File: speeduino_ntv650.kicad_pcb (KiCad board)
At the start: 2 copper layers, 101.6 x 96.5 mm, 70 parts, among them IC1 SP721, IC2 TC4424, J1 Conn_01x25_DB-25, P1 MAX9926_9927, Q1 STP62NS04Z, Q2 STP62NS04Z, Q3 STP62NS04Z, U1 LM2937xT

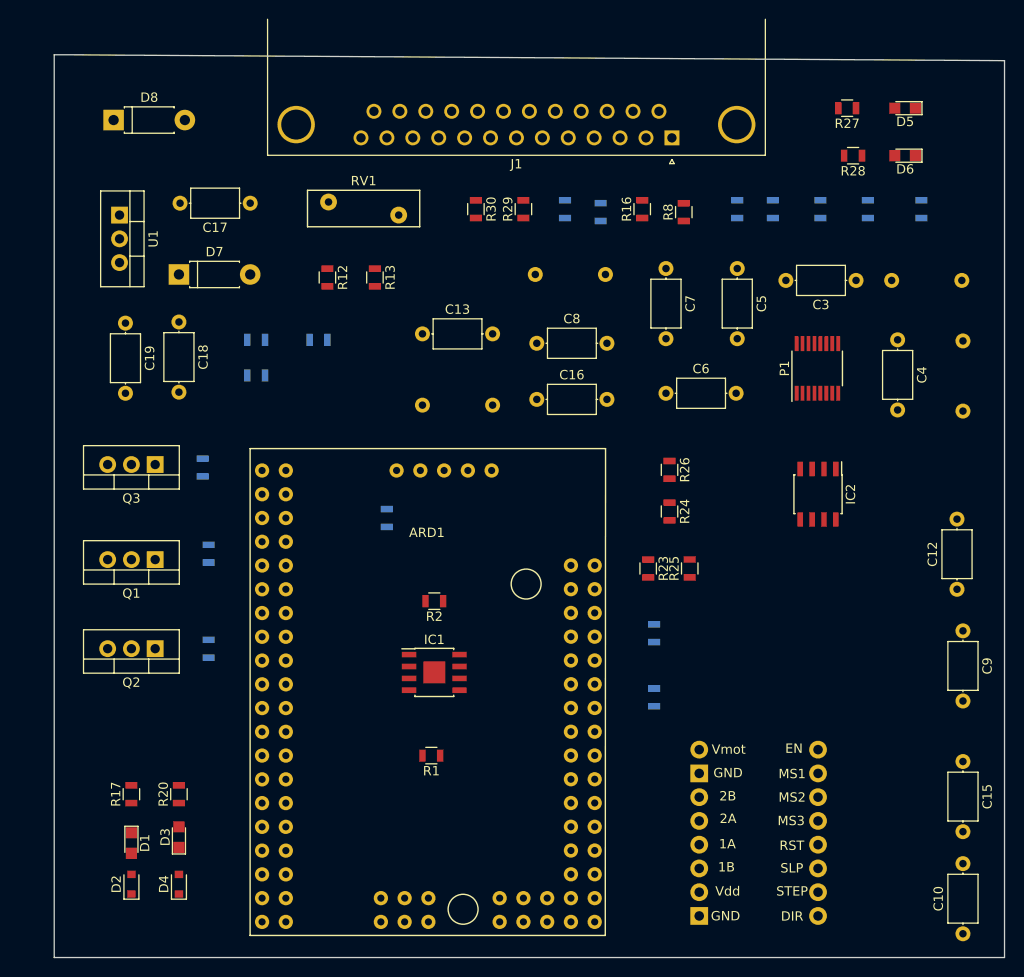
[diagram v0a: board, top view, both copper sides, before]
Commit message: change footprints
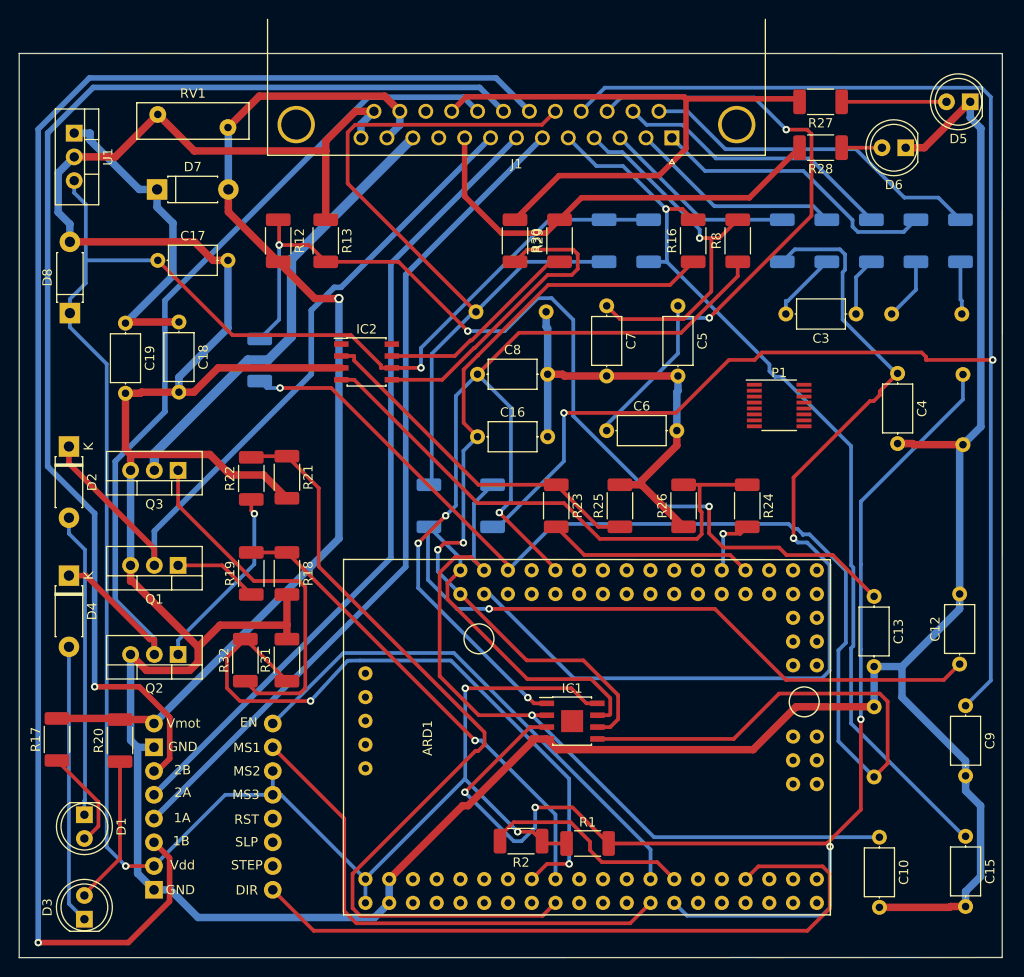
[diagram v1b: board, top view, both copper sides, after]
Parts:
- D1, D3, D5, D6: footprint LEDs:LED_0805 -> LED_THT:LED_D5.0mm
- D2, D4: footprint Diodes_SMD:D_0805 -> Diode_THT:D_DO-41_SOD81_P7.62mm_Horizontal
- R1, R10, R11, R12, R13, R14, R15, R16, R17, R2, R20, R23, R24, R25, R26, R27, R28, R29, R3, R30, R4, R5, R6, R7, R8, R9: footprint Resistors_SMD:R_0805 -> Resistor_SMD:R_2010_5025Metric
- R18, R19, R21, R22, R31, R32: footprint Resistors_SMD:R_0805 -> Resistor_SMD:R_2010_5025Metric; moved to F.Cu
- moved C14 62.5 mm to (151.8, 103.2), turned to 90 degrees
- moved A1 58.4 mm to (88.8, 96.3)
- moved C13 55.9 mm to (151.8, 83.9), turned to 270 degrees
- moved IC2 50.3 mm to (97.5, 58.9), turned to 0 degrees
- moved D2 47.3 mm to (65.7, 67.9), turned to 270 degrees
- moved D4 35.0 mm to (65.7, 81.7), turned to 270 degrees
- moved ARD1 31.0 mm to (99.9, 104.0), turned to 90 degrees
- moved R31 30.6 mm to (89.0, 90.8), turned to 90 degrees
- moved R11 27.7 mm to (104.2, 74.3)
- moved R2 27.3 mm to (114.0, 110.1)
- moved R9 26.8 mm to (111.0, 74.3)
- moved D8 21.2 mm to (65.8, 53.7), turned to 90 degrees
- moved R32 21.1 mm to (84.6, 90.8), turned to 90 degrees
- moved RV1 20.5 mm to (82.7, 33.8)
- moved R1 19.2 mm to (121.2, 110.4), turned to 0 degrees
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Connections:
- C17 pad 1: 12V -> 5V
- IC2 pad 6: 12V -> 5V
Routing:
- net GND: track 0.00 -> 485.5 mm
- net 5V: track 0.00 -> 240.8 mm, vias 0 -> 4
- net TPS_sens: track 0.00 -> 176.4 mm, vias 0 -> 2
- net STEP-1B-OUT: track 0.00 -> 166.1 mm, vias 0 -> 1
- net ADC-Clamp4: track 0.00 -> 141.6 mm, vias 0 -> 1
- net ADC-Clamp5: track 0.00 -> 137.6 mm, vias 0 -> 4
- net STEP-2B-OUT: track 0.00 -> 129.1 mm, vias 0 -> 1
- net 12V: track 0.00 -> 112.8 mm, vias 0 -> 1
- net ADC-Clamp1: track 0.00 -> 103.5 mm, vias 0 -> 4
- net Net-(C13-Pad1): track 0.00 -> 103.4 mm, vias 0 -> 3
- net MAP-CPU-A3: track 0.00 -> 102.6 mm, vias 0 -> 1
- net ADC-Clamp6: track 0.00 -> 102.3 mm, vias 0 -> 1
- net CLT_sens: track 0.00 -> 100.0 mm, vias 0 -> 1
- net inj-2-out: track 0.00 -> 98.4 mm
- net STEP-1A-OUT: track 0.00 -> 90.0 mm
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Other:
- board size 101.6 x 96.5 mm -> 105.1 x 96.7 mm
- net class 5v_small added: clearance 0.11, trace_width 0.4, via_dia 0.8, via_drill 0.4
